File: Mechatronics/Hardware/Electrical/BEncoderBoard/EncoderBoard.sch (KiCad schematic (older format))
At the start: 50 parts, among them IC1 RN4020-V_RM120, IC2 TP4056, IC3 DW01+G, J1 Conn_01x07_Male, J2 GNDPWR, J4 Barrel_Jack_Switch, J5 Batt+, J7 Batt-, Q1 FS8205, Q2 Q_PMOS_GSD, Q3 Q_PMOS_GSD, U1 STM32F103C8T6, U2 ITR1802, U3 ITR1802, U5 SSD1306OLED, U6 LTC3240, Y1 8Mhz

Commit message: Added changes
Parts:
- removed D2: D, Diode_THT:D_DO-201AD_P5.08mm_Vertical_AnodeUp, symbol Device:D
- removed Q1: FS8205, Encoder:Sot-23(6), symbol Encoder:FS8205
- added Q1: DMosfet, Encoder:Sot-23(6), symbol Encoder:DMosfet
- added U4: 82402305, Encoder:Sot-23(6), symbol Encoder:82402305
- U1: Campo4 Unavailable -> (none); Campo5 None -> (none); Campo6 Mainstream Performance line, ARM Cortex-M3 MCU with 64 Kbyt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 -> (none); Campo7 STMicroelectronics -> (none); Campo8 LQFP-48 STMicroelectronics -> (none); Field4 (none) -> Unavailable; Field5 (none) -> None; Field6 (none) -> Mainstream Performance line, ARM Cortex-M3 MCU with 64 Kbyt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; Field7 (none) -> STMicroelectronics; Field8 (none) -> LQFP-48 STMicroelectronics
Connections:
- wire segments 179 -> 178
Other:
- moved on the sheet: C11, C12, C13, C14, C15, C16, C17, C18, D1, IC1, IC2, IC3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

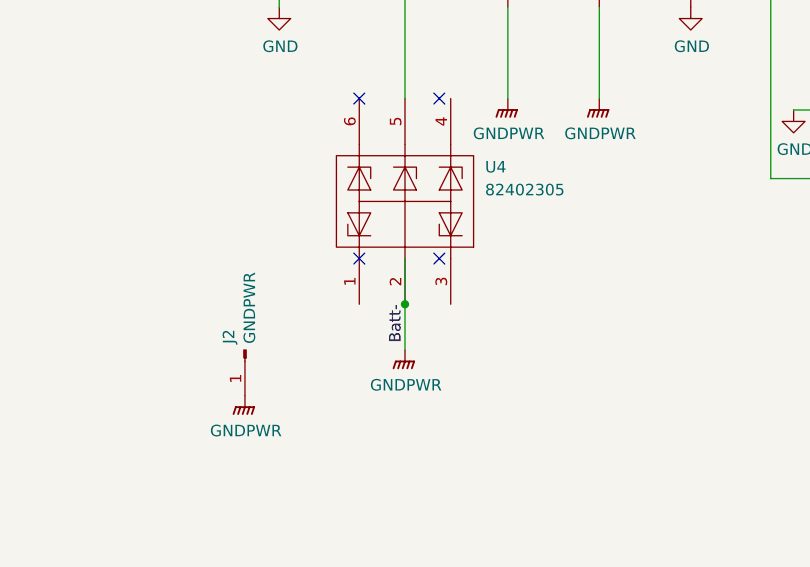
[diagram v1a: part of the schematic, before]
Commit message: Added changes
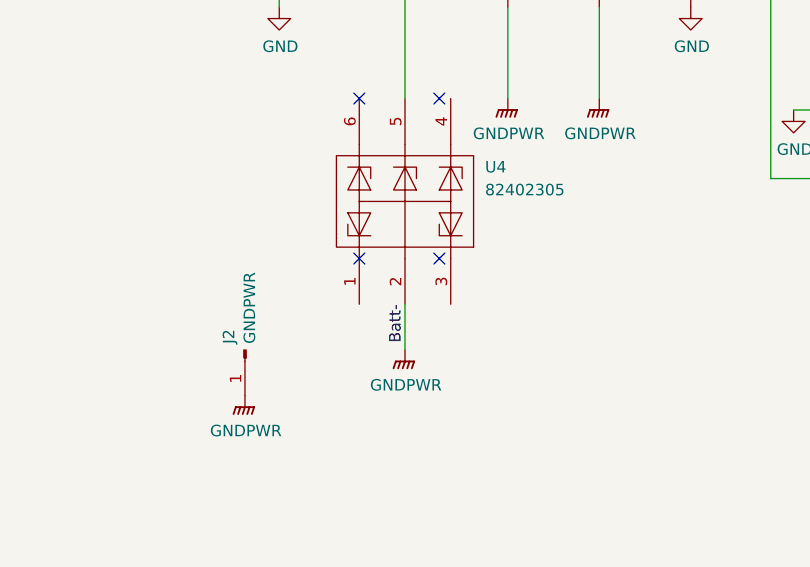
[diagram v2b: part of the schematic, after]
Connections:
- wire segments 178 -> 177
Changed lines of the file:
@@
 Batt-
 Wire Wire Line
-	2800 7150 2800 7350
-Wire Wire Line
 	2800 7350 2800 7550
-Connection ~ 2800 7350
 Wire Wire Line
 	8950 6700 9150 6700
